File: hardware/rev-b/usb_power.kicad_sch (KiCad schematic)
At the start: 11 parts, among them U4 AP2112K-3.3, U5 MCP73831-2-OT

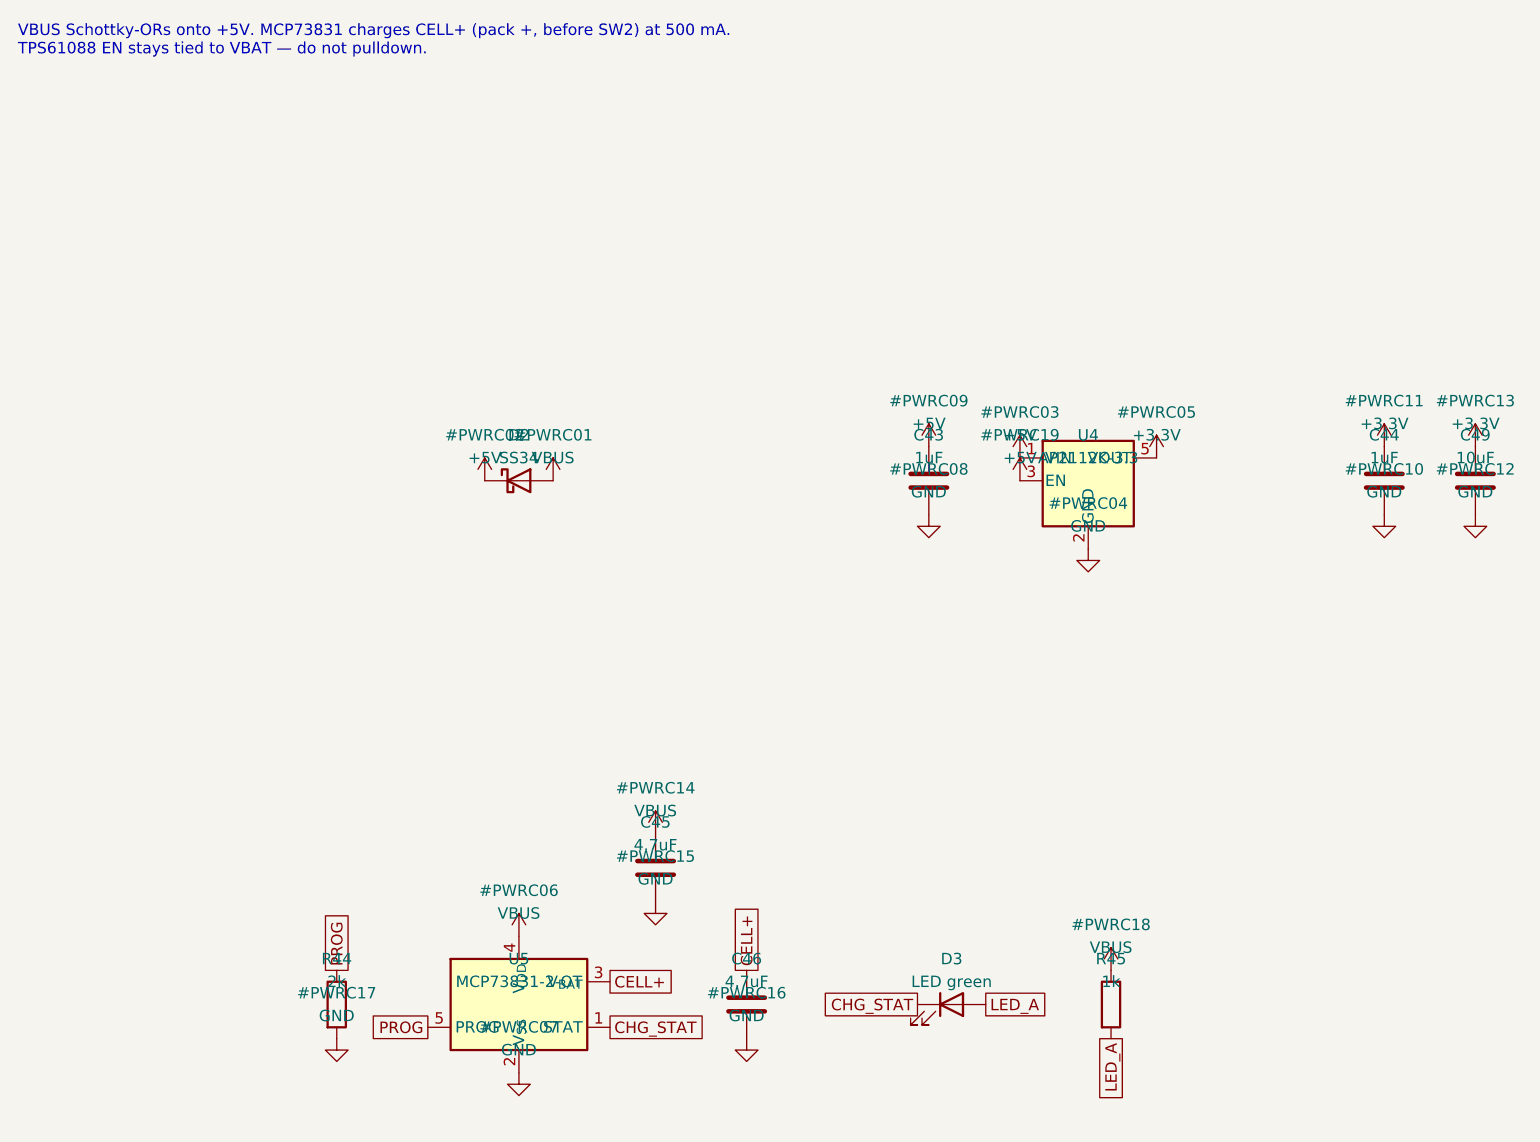
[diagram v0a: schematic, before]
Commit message: update rev-b
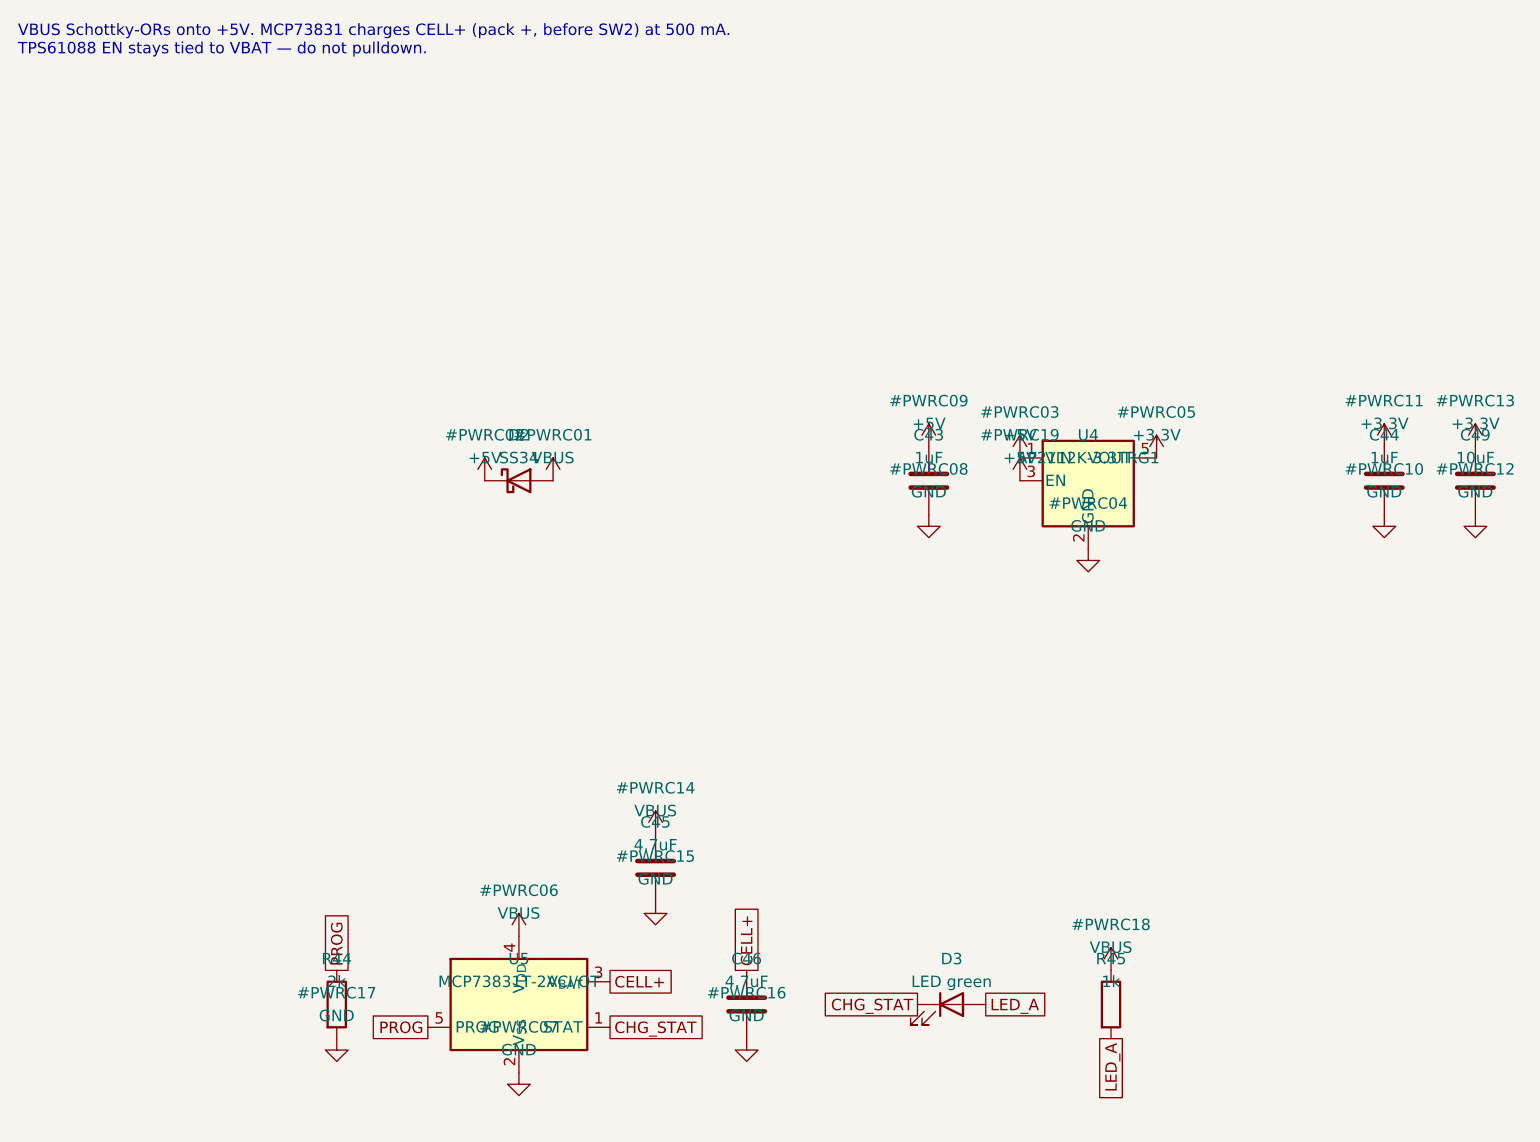
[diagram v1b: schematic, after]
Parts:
- C43, C44, C45, C46: footprint Capacitor_SMD:C_0805_2012Metric_Pad1.18x1.45mm_HandSolder -> Capacitor_SMD:C_0402_1005Metric
- C49: footprint Capacitor_SMD:C_0805_2012Metric_Pad1.18x1.45mm_HandSolder -> Capacitor_SMD:C_0603_1608Metric
- D3: footprint LED_SMD:LED_0805_2012Metric -> LED_SMD:LED_0402_1005Metric
- R44, R45: footprint Resistor_SMD:R_0805_2012Metric_Pad1.20x1.40mm_HandSolder -> Resistor_SMD:R_0201_0603Metric
- U4: value AP2112K-3.3 -> AP2112K-3.3TRG1
- U5: value MCP73831-2-OT -> MCP73831T-2ACI/OT
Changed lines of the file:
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@@
 			)
 		)
-		(property "Footprint" "Capacitor_SMD:C_0805_2012Metric_Pad1.18x1.45mm_HandSolder"
+		(property "Footprint" "Capacitor_SMD:C_0402_1005Metric"
 			(at 172.72 71.12 0)
 			(hide yes)
@@
 			)
 		)
-		(property "Footprint" "Resistor_SMD:R_0805_2012Metric_Pad1.20x1.40mm_HandSolder"
+		(property "Footprint" "Resistor_SMD:R_0201_0603Metric"
 			(at 55.88 129.54 0)
 			(hide yes)
@@
 			)
 		)
-		(property "Value" "MCP73831-2-OT"
+		(property "Value" "MCP73831T-2ACI/OT"
 			(at 76.2 127 0)
 			(show_name no)
@@
 			)
 		)
-		(property "Footprint" "LED_SMD:LED_0805_2012Metric"
+		(property "Footprint" "LED_SMD:LED_0402_1005Metric"
 			(at 124.46 129.54 0)
 			(hide yes)
@@
 			)
 		)
-		(property "Footprint" "Capacitor_SMD:C_0805_2012Metric_Pad1.18x1.45mm_HandSolder"
+		(property "Footprint" "Capacitor_SMD:C_0402_1005Metric"
 			(at 91.44 114.3 0)
 			(hide yes)
@@
 			)
 		)
-		(property "Footprint" "Capacitor_SMD:C_0805_2012Metric_Pad1.18x1.45mm_HandSolder"
+		(property "Footprint" "Capacitor_SMD:C_0603_1608Metric"
 			(at 182.88 71.12 0)
 			(hide yes)
@@
 			)
 		)
-		(property "Footprint" "Capacitor_SMD:C_0805_2012Metric_Pad1.18x1.45mm_HandSolder"
+		(property "Footprint" "Capacitor_SMD:C_0402_1005Metric"
 			(at 121.92 71.12 0)
 			(hide yes)
@@
 			)
 		)
-		(property "Value" "AP2112K-3.3"
+		(property "Value" "AP2112K-3.3TRG1"
 			(at 139.7 68.58 0)
 			(show_name no)
@@
 			)
 		)
-		(property "Footprint" "Resistor_SMD:R_0805_2012Metric_Pad1.20x1.40mm_HandSolder"
+		(property "Footprint" "Resistor_SMD:R_0201_0603Metric"
 			(at 142.24 129.54 0)
 			(hide yes)
@@
 			)
 		)
-		(property "Footprint" "Capacitor_SMD:C_0805_2012Metric_Pad1.18x1.45mm_HandSolder"
+		(property "Footprint" "Capacitor_SMD:C_0402_1005Metric"
 			(at 101.6 129.54 0)
 			(hide yes)
